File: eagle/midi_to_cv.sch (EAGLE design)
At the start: 76 parts, among them IC1 TL084P, IC2 TL084P, IC3 TL084P, IC4 TL084P, IC5 TL084P, U1 ATMEGA328P_PDIP

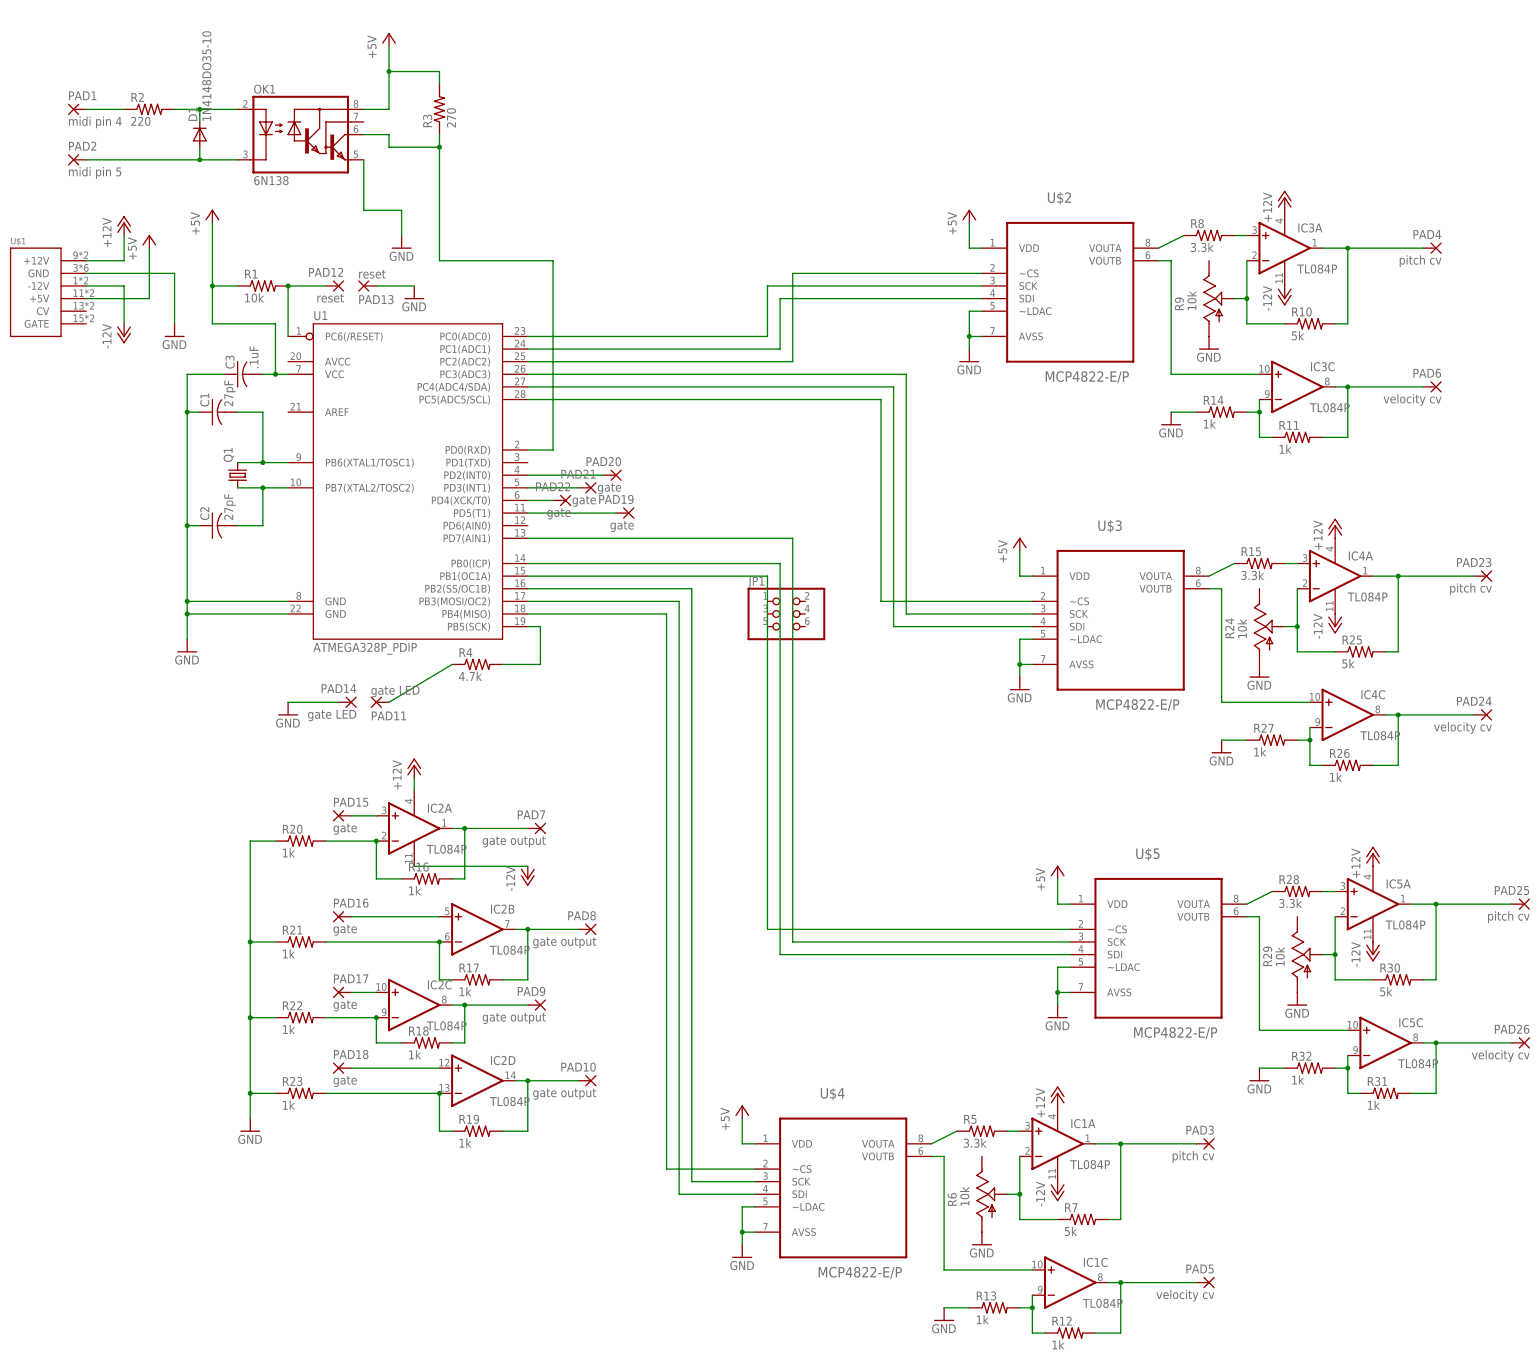
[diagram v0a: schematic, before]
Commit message: prettied up the schematic
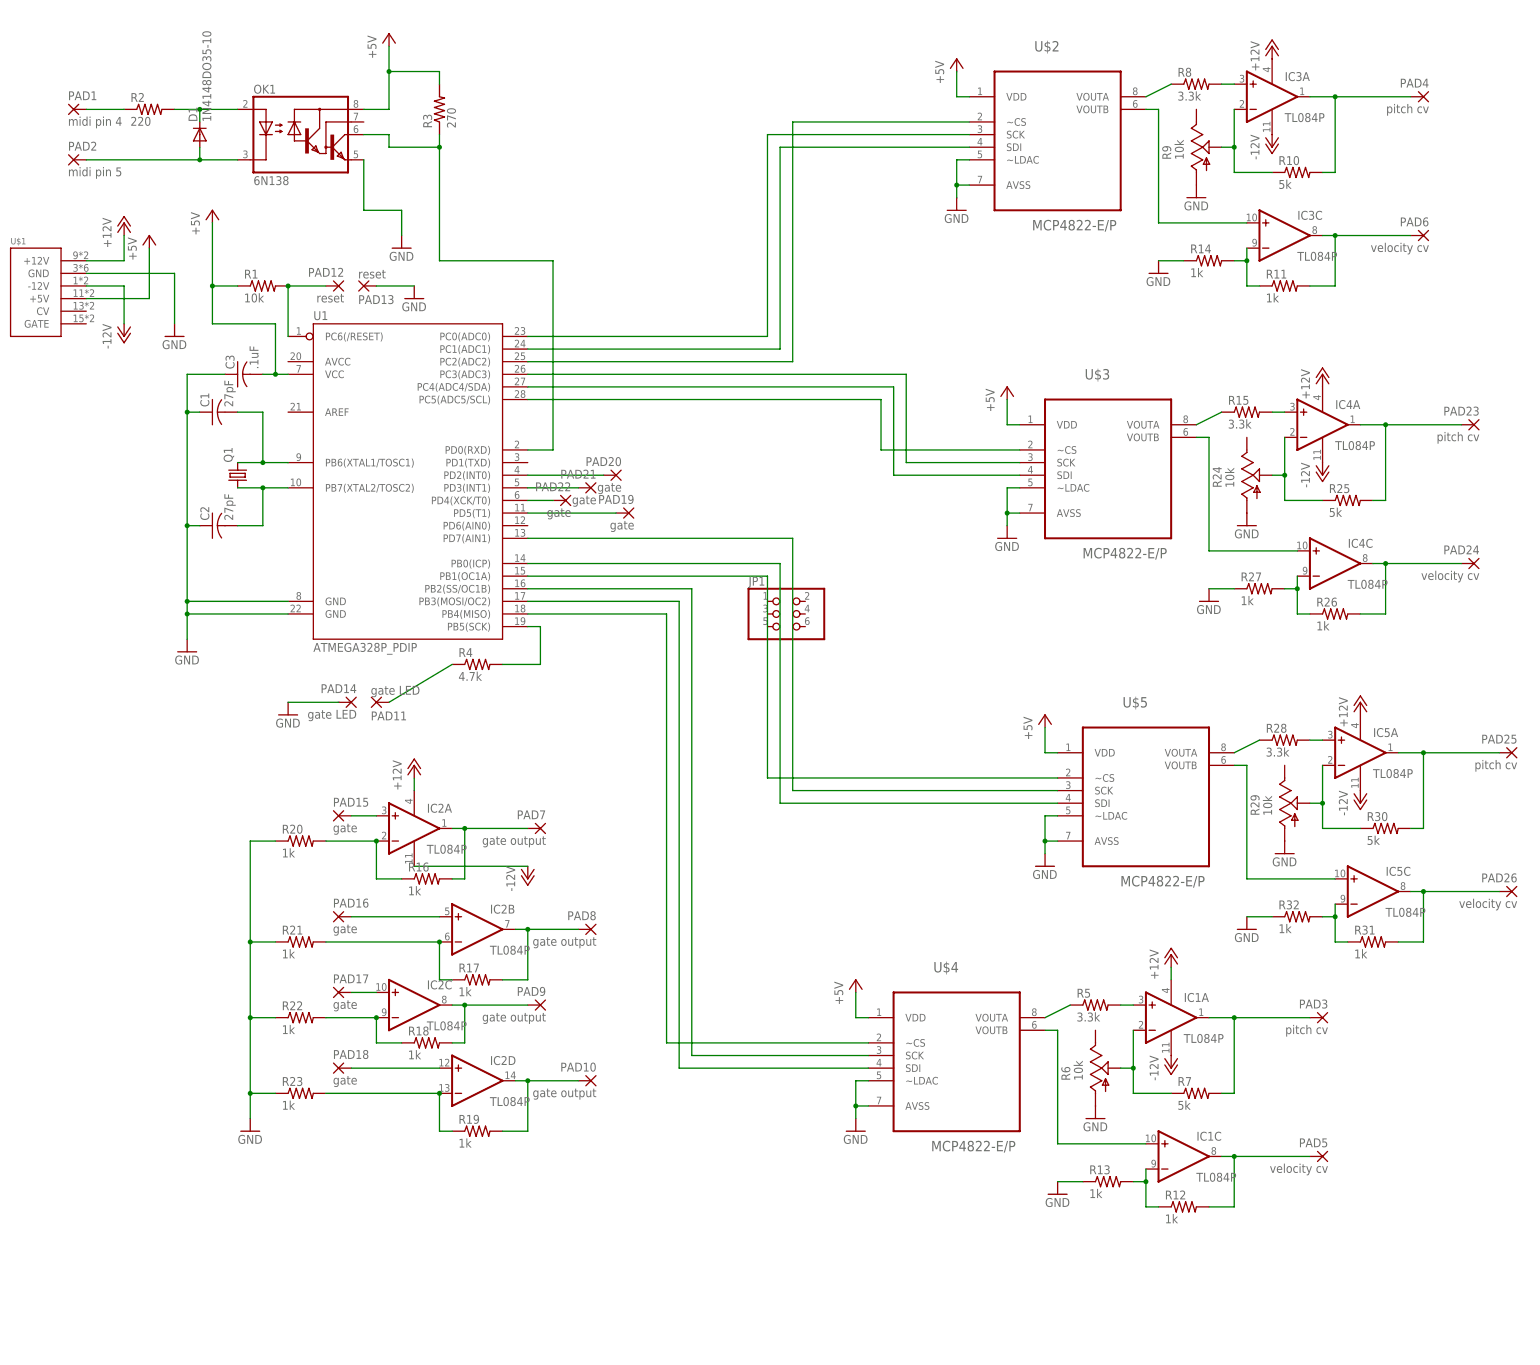
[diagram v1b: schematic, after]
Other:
- moved on the sheet: IC1A, IC1C, IC3A, IC3C, IC4A, IC4C, IC5A, IC5C, PAD23, PAD24, PAD25, PAD26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
